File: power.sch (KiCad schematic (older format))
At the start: 32 parts, among them U1 MCP1603L, U2 MCP16311/2, U3 MCP16311/2

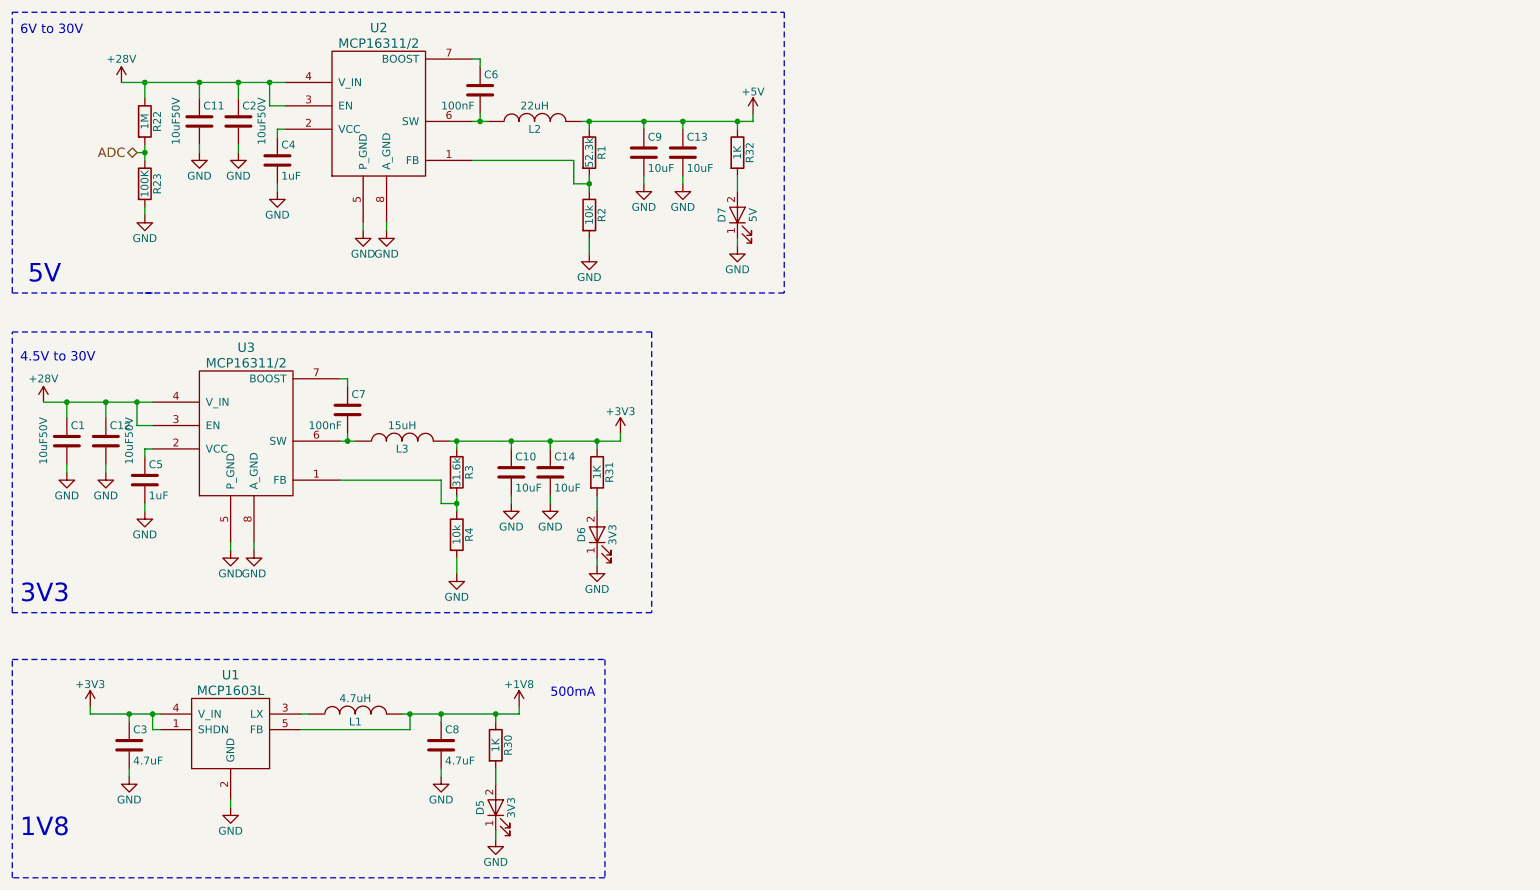
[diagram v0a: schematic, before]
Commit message: beta
beta pcb version 0.001V
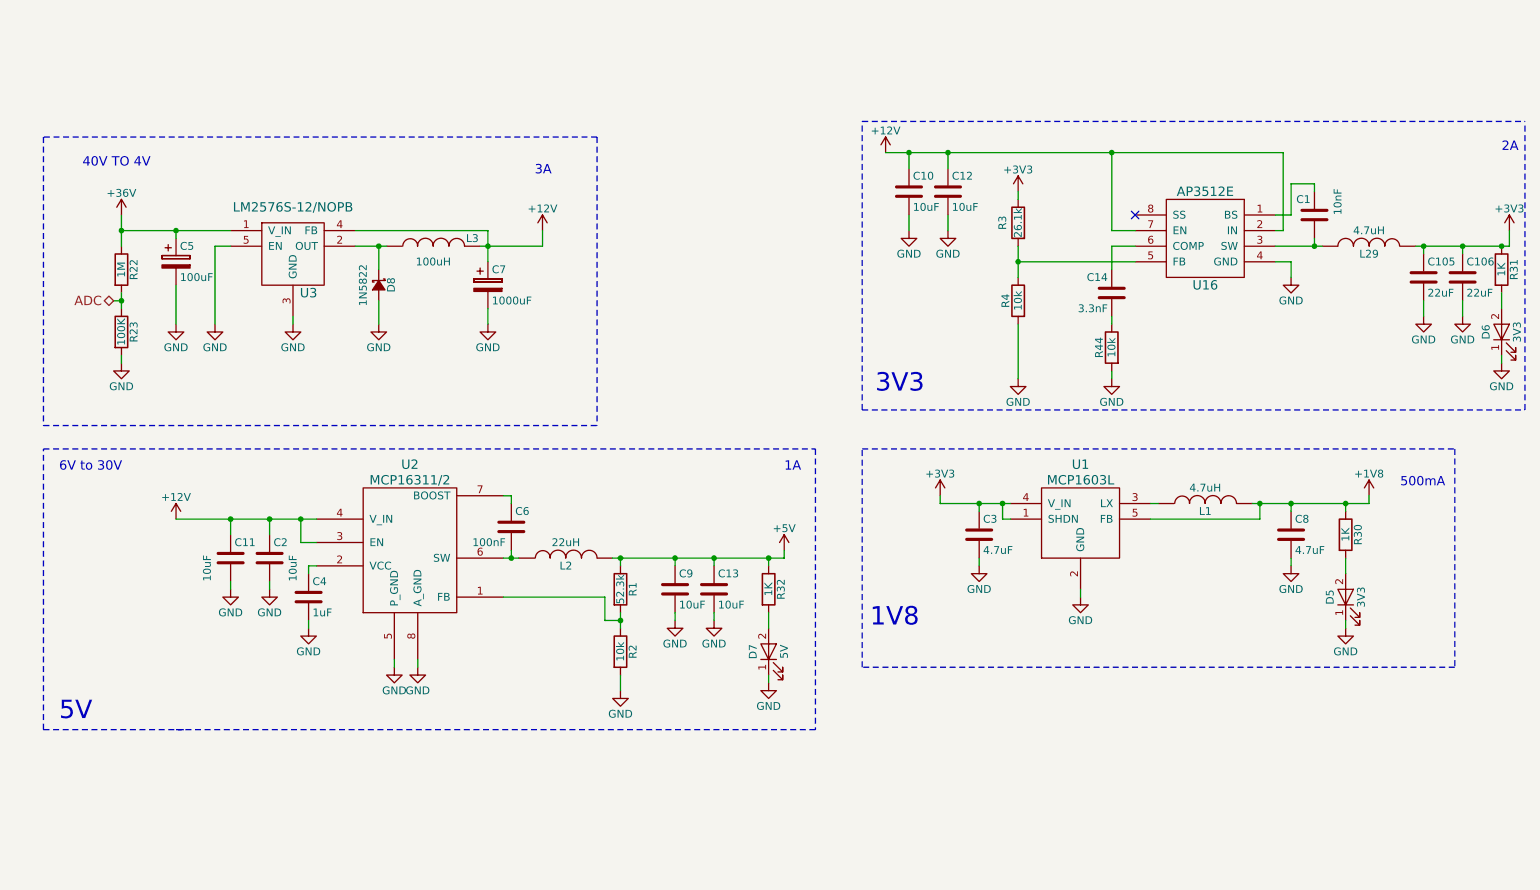
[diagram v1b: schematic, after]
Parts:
- removed C5: 1uF, Capacitors_SMD:C_0402, symbol C
- removed C7: 100nF, Capacitors_SMD:C_0402, symbol C
- removed U3: MCP16311/2, Housings_SSOP:MSOP-8-1EP_3x3mm_Pitch0.65mm, symbol MCP16311/2-RESCUE-autonomous_rc_pcb
- added C105, C106: 22uF, Capacitors_SMD:C_0805_HandSoldering, symbol C
- added C5: 100uF, Capacitor_THT:CP_Radial_D8.0mm_P3.50mm, symbol CP
- added C7: 1000uF, Capacitor_THT:CP_Radial_D8.0mm_P5.00mm, symbol CP
- added D8: 1N5822, PAUL-DIODE-SMD:D_DO-201AD_P5.08mm_Vertical_AnodeUp, symbol Schottky
- added L29: 4.7uH, Inductors_SMD:L_Taiyo-Yuden_NR-50xx_HandSoldering, symbol INDUCTOR
- added R44: 10k, Resistor_SMD:R_0402_1005Metric, symbol R
- added U16: AP3512E, Package_SO:PowerIntegrations_SO-8, symbol AP3512E
- added U3: LM2576S-12/NOPB, Package_TO_SOT_SMD:TO-263-5_TabPin3, symbol LM2576S-12/NOPB
- C1: value 10uF50V -> 10nF
- C10: footprint Capacitors_SMD:C_0402 -> Capacitors_SMD:C_0805_HandSoldering
- C11, C2: value 10uF50V -> 10uF
- C12: value 10uF50V -> 10uF; footprint Capacitors_SMD:C_0402 -> Capacitors_SMD:C_0805_HandSoldering
- C14: value 10uF -> 3.3nF
- L3: value 15uH -> 100uH; footprint Inductors_SMD:L_Abracon_ASPI-3012S -> Inductors_SMD:L_Vishay_IHLP-4040; MPN VLCF4020T-150MR68 -> MSS1210-104KED
- R3: value 31.6k -> 26.1k; footprint Resistors_SMD:R_0402 -> Resistor_SMD:R_0402_1005Metric
- R4: footprint Resistors_SMD:R_0402 -> Resistor_SMD:R_0402_1005Metric
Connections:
- net +3V3: now also C105.1, C106.1, L29.1; no longer C10.1, C14.1, L3.2
- net GND: now also C105.2, C106.2, C5.2, C7.2, D8.A, R44.2, U16.4 (GND), U3.3 (GND), U3.5 (EN); no longer C1.2, C14.2
- net at L3.1: now also D8.K, U3.2 (OUT)
- net at R3.2, R4.1: now also U16.5 (FB)
- net +28V renamed +12V
- net +12V: now also C10.1, L3.2, C7.1, U16.2 (IN), U16.7 (EN), U3.4 (FB); no longer C1.1, R22.1
- new net: C1.1, U16.1 (BS)
- new net: C1.2, L29.2, U16.3 (SW)
- new net: C14.1, U16.6 (COMP)
- new net: C14.2, R44.1
- new net +36V: C5.1, R22.1, U3.1 (V_IN)
- no-connect marks 0 -> 1
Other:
- note added: "1A\n"
- note added: "2A\n"
- note added: "3A\n"
- note added: "40V TO 4V \n"
- note removed: "4.5V to 30V\n"
- moved on the sheet: C1, C11, C13, C2, C3, C4, C6, C8, C9, D5, D6, D7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
